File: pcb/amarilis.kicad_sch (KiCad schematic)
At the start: 0 parts

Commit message: schematics done
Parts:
- added D1, D10, D11, D12, D13, D14, D15, D16, D17, D18, D19, D2, D20, D21, D22, D23, D24, D25, D26, D27, D28, D29, D3, D30, D31, D32, D33, D34, D35, D36, D4, D5, D6, D7, D8, D9: 1N4148, Diode_THT:D_DO-35_SOD27_P7.62mm_Horizontal, symbol Diode:1N4148
- added RZ1: RP2040-Zero, RP2040-Zero-Kicad:RP2040-Zero, symbol rp2040-zero:RP2040-Zero
- added SW1, SW10, SW11, SW12, SW13, SW14, SW15, SW16, SW17, SW18, SW19, SW2, SW20, SW21, SW22, SW23, SW24, SW25, SW26, SW27, SW28, SW29, SW3, SW30, SW31, SW32, SW33, SW34, SW35, SW36, SW4, SW5, SW6, SW7, SW8, SW9: SW_PUSH, symbol kbd:SW_PUSH
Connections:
- new net: D27.2 (A), SW27.2
- new net: D26.2 (A), SW26.2
- new net: D21.2 (A), SW21.2
- new net: D3.2 (A), SW3.2
- new net: D14.2 (A), SW14.2
- new net: D1.2 (A), SW1.2
- new net: D32.2 (A), SW32.2
- new net: D9.2 (A), SW9.2
- new net: D13.2 (A), SW13.2
- new net: D8.2 (A), SW8.2
- new net: D16.2 (A), SW16.2
- new net: D12.2 (A), SW12.2
- new net: D24.2 (A), SW24.2
- new net: D28.2 (A), SW28.2
- new net: D34.2 (A), SW34.2
- new net: D7.2 (A), SW7.2
- new net: D35.2 (A), SW35.2
- new net: D19.2 (A), SW19.2
- new net: D20.2 (A), SW20.2
- new net: D25.2 (A), SW25.2
- new net: D2.2 (A), SW2.2
- new net: D36.2 (A), SW36.2
- new net: D15.2 (A), SW15.2
- new net: D11.2 (A), SW11.2
- new net: D18.2 (A), SW18.2
- new net: D31.2 (A), SW31.2
- new net: D23.2 (A), SW23.2
- new net: D29.2 (A), SW29.2
- new net: D4.2 (A), SW4.2
- new net: D6.2 (A), SW6.2
- new net: D22.2 (A), SW22.2
- new net: D10.2 (A), SW10.2
- new net: D33.2 (A), SW33.2
- new net: D17.2 (A), SW17.2
- new net: D5.2 (A), SW5.2
- new net: D30.2 (A), SW30.2
- new net COL0: RZ1.1 (GP0), SW1.1, SW11.1, SW21.1
- new net COL1: RZ1.2 (GP1), SW12.1, SW2.1, SW22.1
- new net COL2: RZ1.3 (GP2), SW13.1, SW23.1, SW3.1, SW31.1
- new net COL3: RZ1.4 (GP3), SW14.1, SW24.1, SW32.1, SW4.1
- new net COL4: RZ1.5 (GP4), SW15.1, SW25.1, SW33.1, SW5.1
- new net COL5: RZ1.6 (GP5), SW16.1, SW26.1, SW34.1, SW6.1
- new net COL6: RZ1.7 (GP6), SW17.1, SW27.1, SW35.1, SW7.1
- new net COL7: RZ1.8 (GP7), SW18.1, SW28.1, SW36.1, SW8.1
- new net COL8: RZ1.9 (GP8), SW19.1, SW29.1, SW9.1
- new net COL9: RZ1.10 (GP9), SW10.1, SW20.1, SW30.1
- new net ROW0: D1.1 (K), D10.1 (K), D2.1 (K), D3.1 (K), D4.1 (K), D5.1 (K), D6.1 (K), D7.1 (K), D8.1 (K), D9.1 (K), RZ1.11 (GP10)
- new net ROW1: D11.1 (K), D12.1 (K), D13.1 (K), D14.1 (K), D15.1 (K), D16.1 (K), D17.1 (K), D18.1 (K), D19.1 (K), D20.1 (K), RZ1.12 (GP11)
- new net ROW2: D21.1 (K), D22.1 (K), D23.1 (K), D24.1 (K), D25.1 (K), D26.1 (K), D27.1 (K), D28.1 (K), D29.1 (K), D30.1 (K), RZ1.13 (GP12)
- new net ROW3: D31.1 (K), D32.1 (K), D33.1 (K), D34.1 (K), D35.1 (K), D36.1 (K), RZ1.14 (GP13)

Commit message: starting the PCB
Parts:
- D1, D10, D11, D12, D13, D14, D15, D16, D17, D18, D19, D2, D20, D21, D22, D23, D24, D25, D26, D27, D28, D29, D3, D30, D31, D32, D33, D34, D35, D36, D4, D5, D6, D7, D8, D9: footprint Diode_THT:D_DO-35_SOD27_P7.62mm_Horizontal -> kbd:D3_TH
- SW1, SW10, SW11, SW12, SW13, SW14, SW15, SW16, SW17, SW18, SW19, SW2, SW20, SW21, SW22, SW23, SW24, SW25, SW26, SW27, SW28, SW29, SW3, SW30, SW31, SW32, SW33, SW34, SW35, SW36, SW4, SW5, SW6, SW7, SW8, SW9: footprint (none) -> kbd:CherryMX_1u

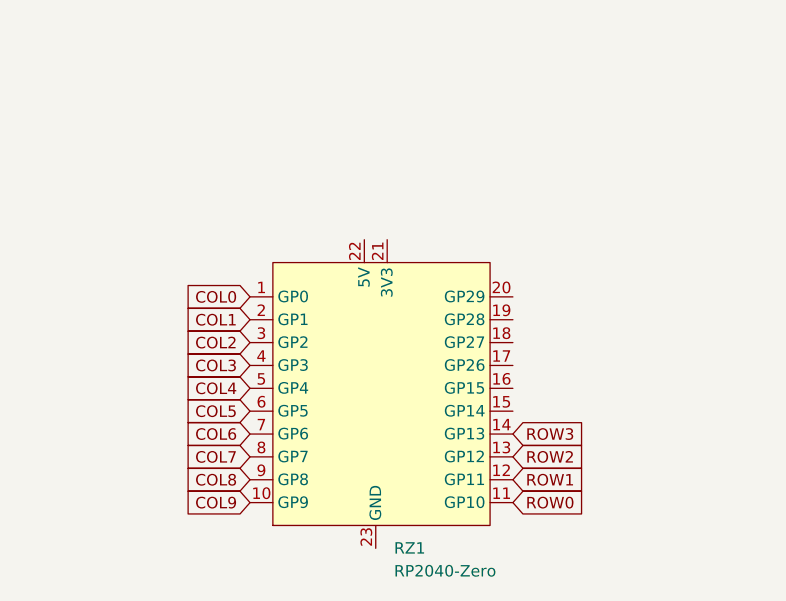
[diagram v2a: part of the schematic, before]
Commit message: PCB ready!
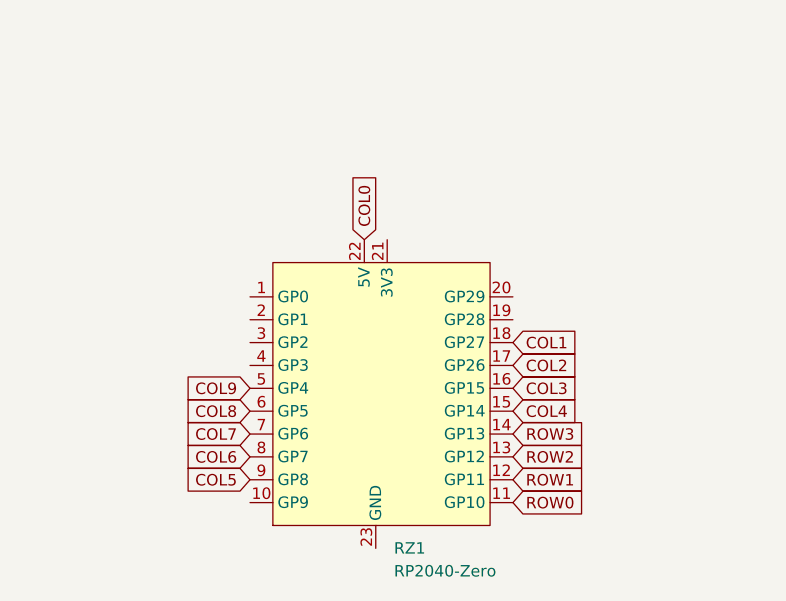
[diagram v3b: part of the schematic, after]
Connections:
- net COL0: now also RZ1.22 (5V); no longer RZ1.1 (GP0)
- net COL1: now also RZ1.18 (GP27); no longer RZ1.2 (GP1)
- net COL2: now also RZ1.17 (GP26); no longer RZ1.3 (GP2)
- net COL3: now also RZ1.16 (GP15); no longer RZ1.4 (GP3)
- net COL4: now also RZ1.15 (GP14); no longer RZ1.5 (GP4)
- net COL5: now also RZ1.9 (GP8); no longer RZ1.6 (GP5)
- net COL6: now also RZ1.8 (GP7); no longer RZ1.7 (GP6)
- net COL7: now also RZ1.7 (GP6); no longer RZ1.8 (GP7)
- net COL8: now also RZ1.6 (GP5); no longer RZ1.9 (GP8)
- net COL9: now also RZ1.5 (GP4); no longer RZ1.10 (GP9)
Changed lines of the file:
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@@
     (stroke (width 0) (type default) (color 0 0 0 0))
   )
-  (global_label "COL9" (shape input) (at 80.01 162.56 180) (fields_autoplaced)
+  (global_label "COL9" (shape input) (at 80.01 149.86 180) (fields_autoplaced)
     (effects (font (size 1.27 1.27)) (justify right))
-    (property "Intersheet References" "${INTERSHEET_REFS}" (id 0) (at 72.7588 162.4806 0)
+    (property "Intersheet References" "${INTERSHEET_REFS}" (id 0) (at 72.7588 149.7806 0)
       (effects (font (size 1.27 1.27)) (justify right) hide)
     )
@@
     )
   )
-  (global_label "COL7" (shape input) (at 80.01 157.48 180) (fields_autoplaced)
+  (global_label "COL7" (shape input) (at 80.01 154.94 180) (fields_autoplaced)
     (effects (font (size 1.27 1.27)) (justify right))
-    (property "Intersheet References" "${INTERSHEET_REFS}" (id 0) (at 72.7588 157.4006 0)
+    (property "Intersheet References" "${INTERSHEET_REFS}" (id 0) (at 72.7588 154.8606 0)
       (effects (font (size 1.27 1.27)) (justify right) hide)
     )
@@
     )
   )
-  (global_label "COL3" (shape input) (at 80.01 147.32 180) (fields_autoplaced)
-    (effects (font (size 1.27 1.27)) (justify right))
-    (property "Intersheet References" "${INTERSHEET_REFS}" (id 0) (at 72.7588 147.2406 0)
-      (effects (font (size 1.27 1.27)) (justify right) hide)
+  (global_label "COL3" (shape input) (at 109.22 149.86 0) (fields_autoplaced)
+    (effects (font (size 1.27 1.27)) (justify left))
+    (property "Intersheet References" "${INTERSHEET_REFS}" (id 0) (at 116.4712 149.9394 0)
+      (effects (font (size 1.27 1.27)) (justify left) hide)
     )
   )
-  (global_label "COL4" (shape input) (at 80.01 149.86 180) (fields_autoplaced)
-    (effects (font (size 1.27 1.27)) (justify right))
-    (property "Intersheet References" "${INTERSHEET_REFS}" (id 0) (at 72.7588 149.7806 0)
-      (effects (font (size 1.27 1.27)) (justify right) hide)
+  (global_label "COL4" (shape input) (at 109.22 152.4 0) (fields_autoplaced)
+    (effects (font (size 1.27 1.27)) (justify left))
+    (property "Intersheet References" "${INTERSHEET_REFS}" (id 0) (at 116.4712 152.4794 0)
+      (effects (font (size 1.27 1.27)) (justify left) hide)
     )
   )
@@
     )
   )
-  (global_label "COL5" (shape input) (at 80.01 152.4 180) (fields_autoplaced)
+  (global_label "COL5" (shape input) (at 80.01 160.02 180) (fields_autoplaced)
     (effects (font (size 1.27 1.27)) (justify right))
-    (property "Intersheet References" "${INTERSHEET_REFS}" (id 0) (at 72.7588 152.3206 0)
+    (property "Intersheet References" "${INTERSHEET_REFS}" (id 0) (at 72.7588 159.9406 0)
       (effects (font (size 1.27 1.27)) (justify right) hide)
     )
@@
     )
   )
-  (global_label "COL1" (shape input) (at 80.01 142.24 180) (fields_autoplaced)
+  (global_label "COL1" (shape input) (at 109.22 144.78 0) (fields_autoplaced)
+    (effects (font (size 1.27 1.27)) (justify left))
+    (property "Intersheet References" "${INTERSHEET_REFS}" (id 0) (at 116.4712 144.8594 0)
+      (effects (font (size 1.27 1.27)) (justify left) hide)
+    )
+  )
+  (global_label "COL8" (shape input) (at 80.01 152.4 180) (fields_autoplaced)
     (effects (font (size 1.27 1.27)) (justify right))
-    (property "Intersheet References" "${INTERSHEET_REFS}" (id 0) (at 72.7588 142.1606 0)
+    (property "Intersheet References" "${INTERSHEET_REFS}" (id 0) (at 72.7588 152.3206 0)
       (effects (font (size 1.27 1.27)) (justify right) hide)
     )
   )
-  (global_label "COL8" (shape input) (at 80.01 160.02 180) (fields_autoplaced)
+  (global_label "COL6" (shape input) (at 80.01 157.48 180) (fields_autoplaced)
     (effects (font (size 1.27 1.27)) (justify right))
-    (property "Intersheet References" "${INTERSHEET_REFS}" (id 0) (at 72.7588 159.9406 0)
-      (effects (font (size 1.27 1.27)) (justify right) hide)
-    )
-  )
-  (global_label "COL6" (shape input) (at 80.01 154.94 180) (fields_autoplaced)
-    (effects (font (size 1.27 1.27)) (justify right))
-    (property "Intersheet References" "${INTERSHEET_REFS}" (id 0) (at 72.7588 154.8606 0)
+    (property "Intersheet References" "${INTERSHEET_REFS}" (id 0) (at 72.7588 157.4006 0)
       (effects (font (size 1.27 1.27)) (justify right) hide)
     )
@@
     )
   )
-  (global_label "COL0" (shape input) (at 80.01 139.7 180) (fields_autoplaced)
-    (effects (font (size 1.27 1.27)) (justify right))
-    (property "Intersheet References" "${INTERSHEET_REFS}" (id 0) (at 72.7588 139.6206 0)
-      (effects (font (size 1.27 1.27)) (justify right) hide)
+  (global_label "COL0" (shape input) (at 92.71 133.35 90) (fields_autoplaced)
+    (effects (font (size 1.27 1.27)) (justify left))
+    (property "Intersheet References" "${INTERSHEET_REFS}" (id 0) (at 92.7894 126.0988 90)
+      (effects (font (size 1.27 1.27)) (justify left) hide)
     )
   )
-  (global_label "COL2" (shape input) (at 80.01 144.78 180) (fields_autoplaced)
-    (effects (font (size 1.27 1.27)) (justify right))
-    (property "Intersheet References" "${INTERSHEET_REFS}" (id 0) (at 72.7588 144.7006 0)
-      (effects (font (size 1.27 1.27)) (justify right) hide)
+  (global_label "COL2" (shape input) (at 109.22 147.32 0) (fields_autoplaced)
+    (effects (font (size 1.27 1.27)) (justify left))
+    (property "Intersheet References" "${INTERSHEET_REFS}" (id 0) (at 116.4712 147.3994 0)
+      (effects (font (size 1.27 1.27)) (justify left) hide)
     )
   )
